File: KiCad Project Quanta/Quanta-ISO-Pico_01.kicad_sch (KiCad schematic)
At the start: 167 parts, among them SW1-1 SW_Push, SW1-10 SW_Push, SW1-11 SW_Push, SW1-12 SW_Push, SW1-13 SW_Push, SW1-2 SW_Push, SW1-3 SW_Push, SW1-4 SW_Push, SW1-5 SW_Push, SW1-6 SW_Push, SW1-7 SW_Push, SW1-8 SW_Push, SW1-9 SW_Push, SW2-1 SW_Push, SW2-10 SW_Push, SW2-11 SW_Push, SW2-12 SW_Push, SW2-13 SW_Push, SW2-14 SW_Push, SW2-15 SW_Push, SW2-2 SW_Push, SW2-3 SW_Push, SW2-4 SW_Push, SW2-5 SW_Push, SW2-6 SW_Push, SW2-7 SW_Push, SW2-8 SW_Push, SW2-9 SW_Push, SW3-1 SW_Push, SW3-10 SW_Push, SW3-11 SW_Push, SW3-12 SW_Push, SW3-13 SW_Push, SW3-14 SW_Push, SW3-15 SW_Push, SW3-2 SW_Push, SW3-3 SW_Push, SW3-4 SW_Push, SW3-5 SW_Push, SW3-6 SW_Push, SW3-7 SW_Push, SW3-8 SW_Push, SW3-9 SW_Push, SW4-1 SW_Push, SW4-10 SW_Push, SW4-11 SW_Push, SW4-12 SW_Push, SW4-13 SW_Push, SW4-14 SW_Push, SW4-2 SW_Push, SW4-3 SW_Push, SW4-4 SW_Push, SW4-5 SW_Push, SW4-6 SW_Push, SW4-7 SW_Push, SW4-8 SW_Push, SW4-9 SW_Push, SW5-1 SW_Push, SW5-10 SW_Push, SW5-11 SW_Push, SW5-12 SW_Push, SW5-13 SW_Push, SW5-14 SW_Push, SW5-15 SW_Push, SW5-2 SW_Push, SW5-3 SW_Push, SW5-4 SW_Push, SW5-5 SW_Push, SW5-6 SW_Push, SW5-7 SW_Push, SW5-8 SW_Push, SW5-9 SW_Push, SW6-1 SW_Push, SW6-10 SW_Push, SW6-2 SW_Push, SW6-3 SW_Push, SW6-4 SW_Push, SW6-5 SW_Push, SW6-6 SW_Push, SW6-7 SW_Push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

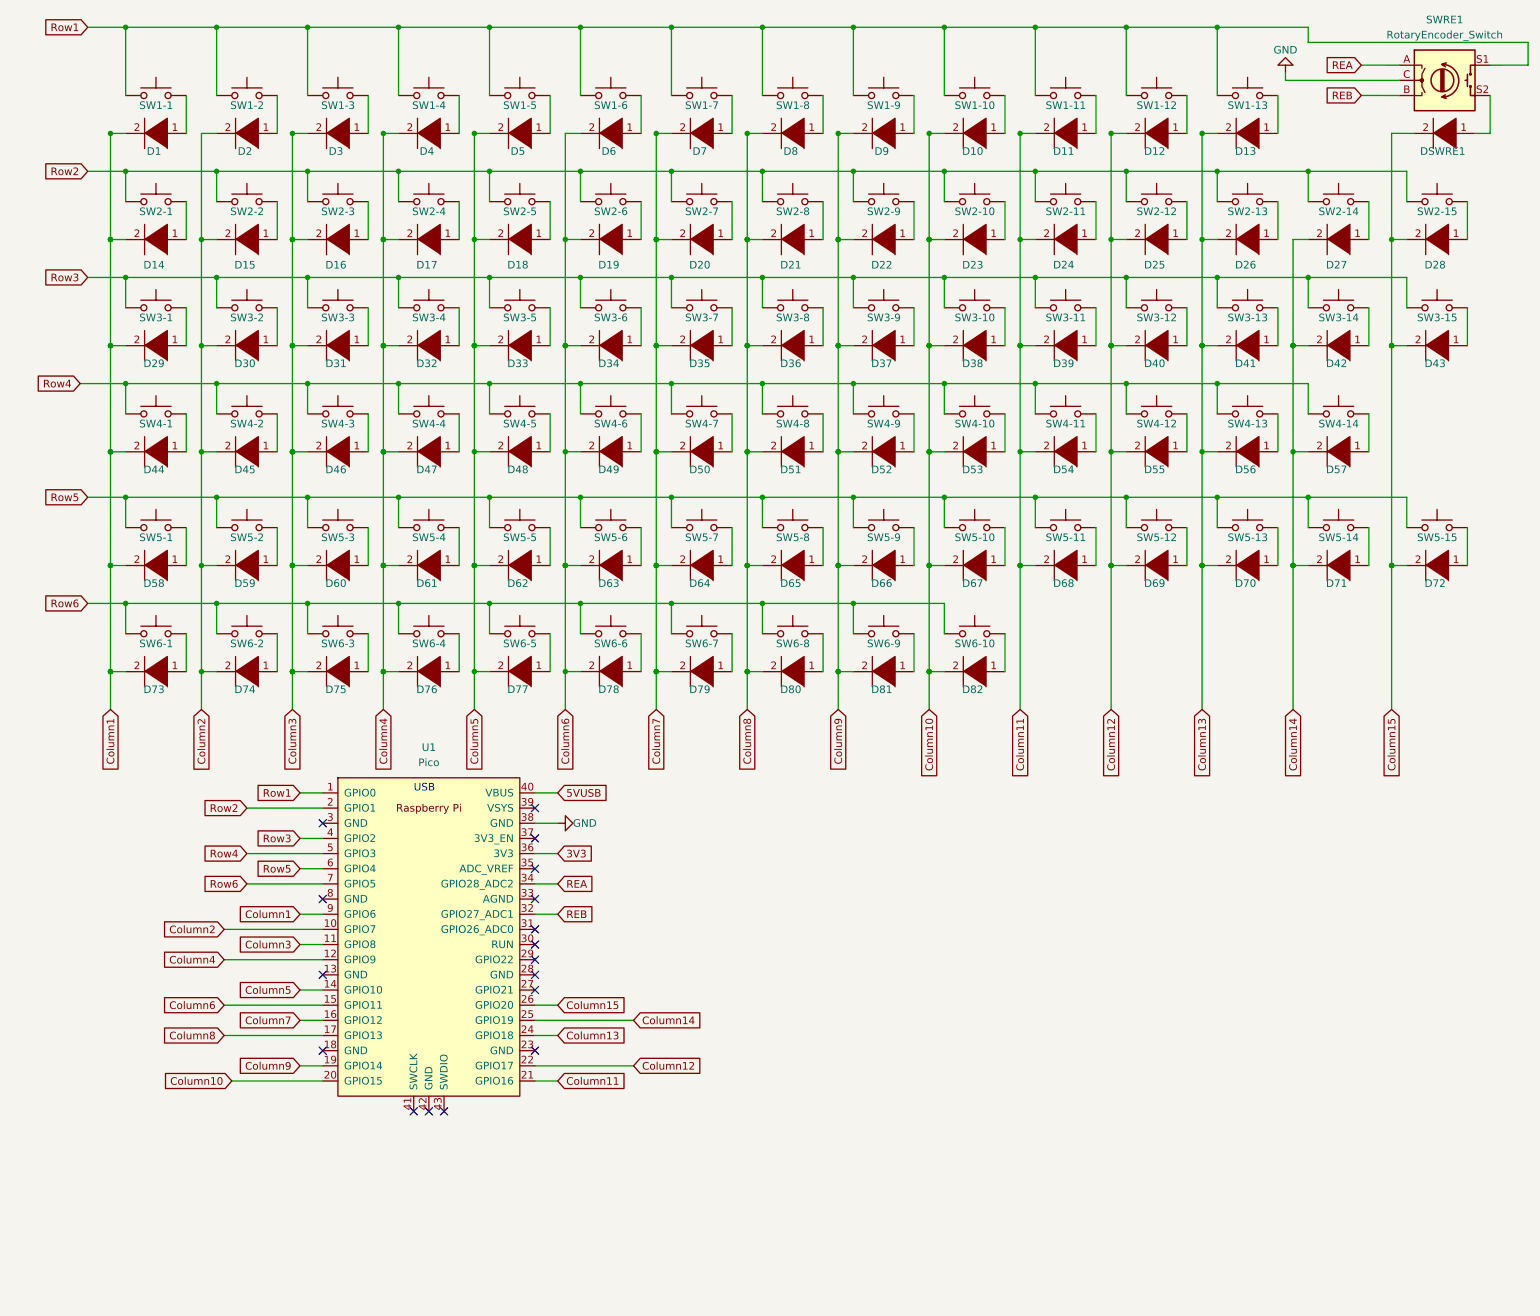
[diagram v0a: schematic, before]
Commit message: new kicad project
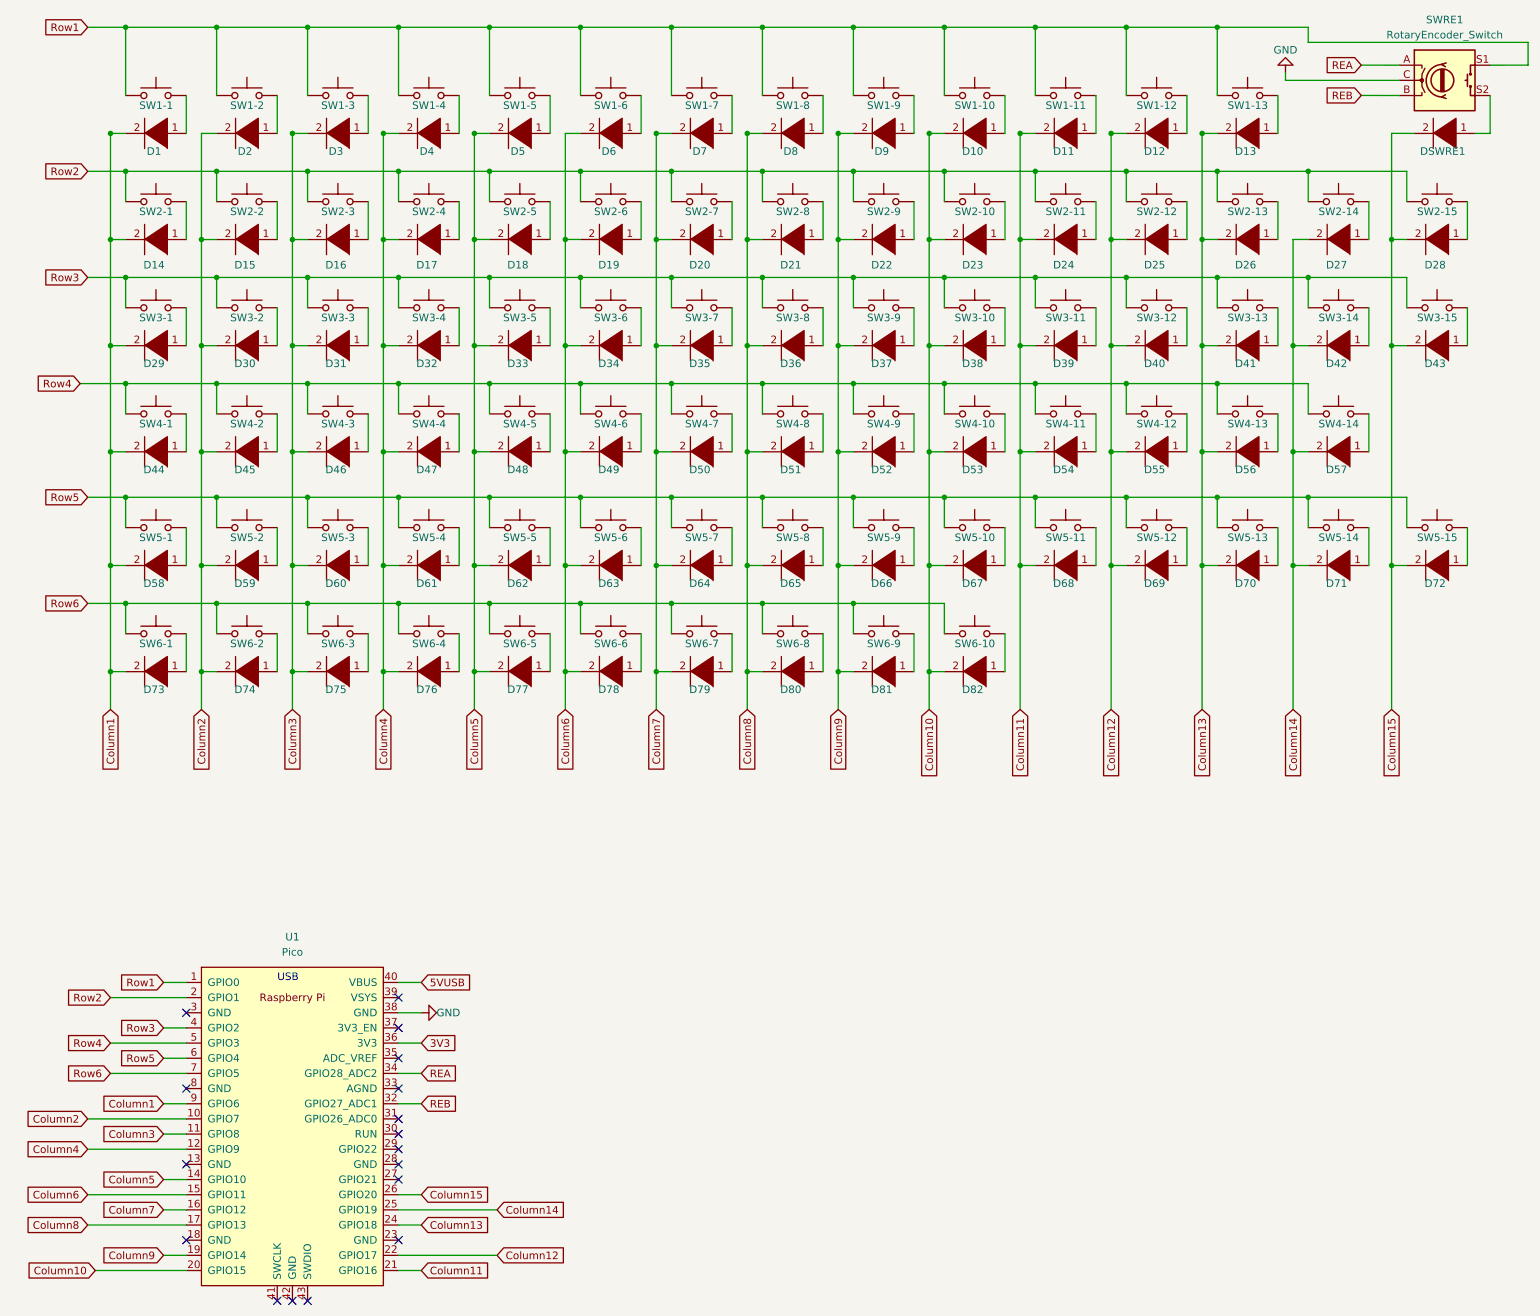
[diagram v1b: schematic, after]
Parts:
- D1, D10, D11, D12, D13, D14, D15, D16, D17, D18, D19, D2, D20, D21, D22, D23, D24, D25, D26, D27, D28, D29, D3, D30, D31, D32, D33, D34, D35, D36, D37, D38, D39, D4, D40, D41, D42, D43, D44, D45, D46, D47, D48, D49, D5, D50, D51, D52, D53, D54, D55, D56, D57, D58, D59, D6, D60, D61, D62, D63, D64, D65, D66, D67, D68, D69, D7, D70, D71, D72, D73, D74, D75, D76, D77, D78, D79, D8, D80, D81, D82, D9, DSWRE1: footprint (none) -> Diode_THT:D_A-405_P7.62mm_Horizontal
- SW1-1, SW1-10, SW1-11, SW1-12, SW1-13, SW1-2, SW1-3, SW1-4, SW1-5, SW1-6, SW1-7, SW1-8, SW1-9, SW2-1, SW2-10, SW2-11, SW2-12, SW2-13, SW2-14, SW2-15, SW2-2, SW2-3, SW2-4, SW2-5, SW2-6, SW2-7, SW2-8, SW2-9, SW3-1, SW3-10, SW3-11, SW3-12, SW3-13, SW3-14, SW3-15, SW3-2, SW3-3, SW3-4, SW3-5, SW3-6, SW3-7, SW3-8, SW3-9, SW4-1, SW4-10, SW4-11, SW4-12, SW4-13, SW4-14, SW4-2, SW4-3, SW4-4, SW4-5, SW4-6, SW4-7, SW4-8, SW4-9, SW5-1, SW5-10, SW5-11, SW5-12, SW5-13, SW5-14, SW5-15, SW5-2, SW5-3, SW5-4, SW5-5, SW5-6, SW5-7, SW5-8, SW5-9, SW6-1, SW6-10, SW6-2, SW6-3, SW6-4, SW6-5, SW6-6, SW6-7, SW6-8, SW6-9: footprint (none) -> Button_Switch_Keyboard:SW_Cherry_MX_1.00u_PCB
- SWRE1: footprint (none) -> Rotary_Encoder:RotaryEncoder_Bourns_Vertical_PEC12R-3xxxF-Sxxxx
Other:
- moved on the sheet: U1
